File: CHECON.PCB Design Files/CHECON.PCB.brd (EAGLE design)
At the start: 81.7 x 51.6 mm, 73 parts

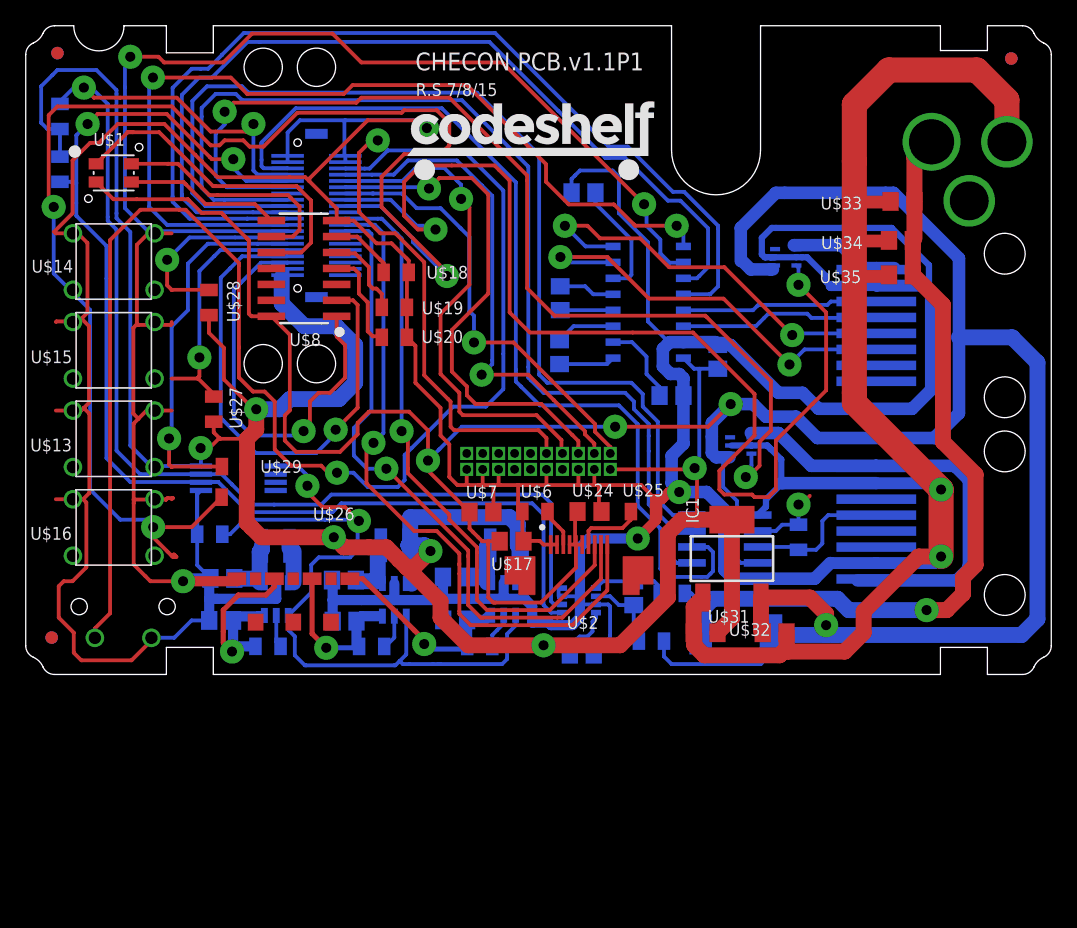
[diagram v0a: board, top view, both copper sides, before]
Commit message: New CHE
Starting on new CHE
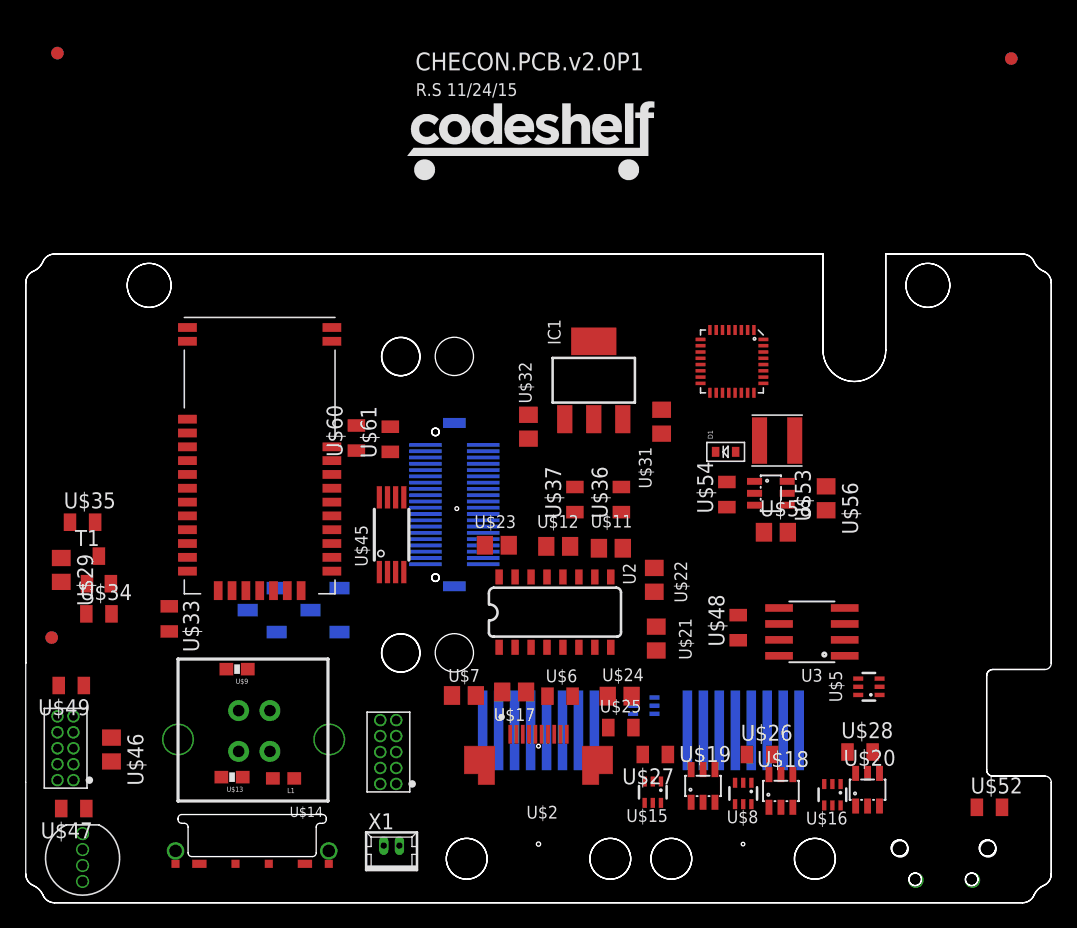
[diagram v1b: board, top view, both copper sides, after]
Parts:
- removed C11, C14: 0.1uF, GW-devices:C0805
- removed LQH3NPN100NM0L: 1212_IND, KW2:1212_IND
- removed R10: (no value), GW-devices:R2512
- removed R12, R13: 10, GW-devices:RF-C0805
- removed U$59: BL_CON, KW2:009155004301006
- removed U$62: INA219B, KW2:DCN-R-PDSO-G8
- added D1: (no value), adafruit:SOD-523
- added JP1, JP2: (no value), KW2:2X5HDR
- added L1: (no value), SparkFun:0603
- added T1: BC849, transistor:SOT23
- added X1: 53047-02, con-molex:53047-02
- U$1: value RGLBED -> 2.7_BL_CONN; device KW2:RGBLED -> KW2:XD2B-0406-26A
- U$13: value SWITCH-TACTILE-FSM -> TVS0603; device GW-devices:SWITCH-TACTILE-FSM -> SparkFun:0603-RES
- U$14: value SWITCH-TACTILE-FSM -> USB_B; device GW-devices:SWITCH-TACTILE-FSM -> KW2:USB-B-PTH-VERTICAL
- U$15, U$16: value SWITCH-TACTILE-FSM -> MIC94061C6; device GW-devices:SWITCH-TACTILE-FSM -> GW-devices:SC70-6L
- U$18, U$19, U$20: value 24 -> BCR401U; device GW-devices:RF-C0805 -> KW2:SOT23-6
- U$26: value 10k -> 40
- U$27, U$28: value 10k -> 15
- U$29: value 10k -> 220pF; device GW-devices:RF-C0805 -> GW-devices:C0805
- U$3: value 2X10JTAG -> KL20; device KW2:2X10JTAG -> KW2:QFN-32
- U$33: value 0.1uF -> 1.5k; device GW-devices:C0805 -> GW-devices:RF-C0805
- U$34: value 1uF -> 4.7k; device GW-devices:C0805 -> GW-devices:RF-C0805
- U$35: value 10uF -> 1.1k; device GW-devices:C0805 -> GW-devices:RF-C0805
- U$36, U$37: value SC4541 -> 10k; device KW2:SOT23-6 -> GW-devices:RF-C0805
- U$4, U$5: value (none) -> MIC94061C6
- U$44: value SC4541 -> LED_PTH_2812; device KW2:SOT23-6 -> KW2:LED_PTH_2812
- U$46: value 10k -> 0.1uF; device GW-devices:RF-C0805 -> GW-devices:C0805
- U$47, U$49: value 1212_IND -> 10k; device KW2:1212_IND -> GW-devices:RF-C0805
- U$50, U$51: value 1uF -> CJS; device GW-devices:C0805 -> KW2:CJS
- U$52: value 1uF -> 10k; device GW-devices:C0805 -> GW-devices:RF-C0805
- U$53: value 1uF -> AP5724; device GW-devices:C0805 -> KW2:SOT23-6
- U$54: value 1uF -> 4.99; device GW-devices:C0805 -> GW-devices:RF-C0805
- U$55: value 1uF -> NR4012T220M; device GW-devices:C0805 -> KW2:NR4012T220M
- U$56: value 6.8 -> 1uF; device GW-devices:RF-C0805 -> GW-devices:C0805
- U$57: value 3.3 -> BM78; device GW-devices:RF-C0805 -> KW2:BM78
- U$58: value 3.3 -> 1uF; device GW-devices:RF-C0805 -> GW-devices:C0805
- U$8: value (none) -> MIC94061C6; device GW-devices:SO14 -> GW-devices:SC70-6L
- U$9: value BARREL_CUI_PJ-002A -> TVS0603; device KW2:BARREL_CUI_PJ-002A -> SparkFun:0603-RES
- U2: value (none) -> MAX232SOIC16
- U3: value (none) -> RS485SOIC
- moved U$34 70.4 mm to (-35.0, -21.0)
- moved U$9 69.4 mm to (-24.0, -25.4), flipped to the top
- moved U$30 68.2 mm to (32.3, -42.2)
- moved U$35 68.1 mm to (-36.3, -13.7)
- moved U$33 67.2 mm to (-29.4, -21.4), turned to 270 degrees
- moved U$28 63.0 mm to (25.6, -32.0), turned to 0 degrees
- moved U$16 61.0 mm to (23.4, -35.4), turned to 180 degrees
- moved SCANNER 56.4 mm to (0.00, -40.5), turned to 0 degrees
- moved U$1 56.1 mm to (-22.8, -40.9), turned to 0 degrees
- moved U$15 55.5 mm to (9.10, -35.2), turned to 180 degrees
- moved U$8 54.5 mm to (16.3, -35.3), turned to 180 degrees
- moved U$20 52.1 mm to (26.2, -35.0)
- moved U$18 51.4 mm to (19.3, -35.1)
- moved U$26 46.6 mm to (17.6, -32.2)
- moved U$55 46.5 mm to (19.0, -7.20), flipped to the top, turned to 180 degrees
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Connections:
- removed net N$24: POSCON.P$1, POSCON.P$8, U$5.1
- new net +5V: IC1.3, U$15.4, U$16.4, U$31.2, U$44.P$2, U$8.4
- new net N$58: JP2.P$10, U$3.19, U$49.2
- net +3V3: now also JP1.P$1, JP2.P$1, U$36.2, U$37.2, U$46.2, U$47.1, U$49.1, U$52.1, U$53.6, U$55.P$2, U$58.2; no longer C14.1, LQH3NPN100NM0L.P$1, U$21.1, U$26.2, U$27.2, U$28.2, U$29.2, U$3.P$1, U$36.3, U$37.3, U$44.3, U$47.P$1, U$49.P$1, U$62.4, U2.16
- net GND: now also JP1.P$3, JP1.P$5, JP2.P$3, JP2.P$5, L1.2, U$1.P$4, U$13.1, U$14.GND, U$15.2, U$15.5, U$16.2, U$16.5, U$18.1, U$19.1, U$20.1, U$29.1, U$44.P$3, U$56.1, U$57.P$1, U$57.P$2, U$57.P$3, U$57.P$31, U$57.P$32, U$57.P$33, U$58.1, U$8.2, U$8.5, U$9.1; no longer C14.2, U$13.P$1, U$13.P$2, U$14.P$1, U$14.P$2, U$15.P$1, U$15.P$2, U$16.P$1, U$16.P$2, U$18.2, U$19.2, U$20.2, U$3.P$15, U$3.P$17, U$3.P$19, U$3.P$3, U$3.P$5, U$3.P$9, U$33.1, U$34.1, U$36.2, U$37.2, U$44.2, U$50.1, U$51.1, U$52.1, U$55.2, U$59.P$4, U$62.3, U$62.7, U$62.8, U$8.7, U$9.P$2
- net N$1: now also JP1.P$2, U$50.P$1; no longer U$3.P$2
- net N$11: now also U$33.2, U$34.2; no longer U$8.1
- net N$13: now also U$16.1, U$20.4, U$28.1; no longer U$18.1, U$8.6
- net N$14: now also U$15.1, U$19.4, U$27.1; no longer U$19.1, U$8.5
- net N$15: now also U$18.4, U$26.1, U$8.1; no longer U$20.1, U$8.4
- net N$16: now also T1.2; no longer U$8.2
- net N$2: now also U$45.2, U$53.4; no longer U$10.P$12, U$3.P$6
- net N$25: now also U$21.1, U2.16
- net N$3: now also U$53.3, U$54.1, X1.2; no longer U$10.P$10, U$3.P$8
- net N$35: now also U$14.D-, U$3.4, U$9.2; no longer U$10.P$31, U$15.P$4, U$27.1
- net N$36: now also U$13.2, U$14.D+, U$3.3; no longer U$10.P$27, U$14.P$4, U$28.1
- net N$37: now also U$20.6, U$28.2; no longer U$10.P$29, U$13.P$4, U$29.1
- net N$39: now also U$36.1
- net N$4: now also JP1.P$4, U$51.P$1; no longer U$3.P$4
- net N$40: now also U$37.1
- net N$42: now also U$19.6, U$27.2; no longer U$10.P$18, U$16.P$4, U$26.1
- net N$43: now also U$18.6, U$26.2; no longer U$36.4, U$37.4, U$44.4, U$45.1, U$46.2
- net N$44: now also U$16.3, U$45.1, U$8.3; no longer U$37.1, U$47.P$2, U$50.2
- net N$45: no longer U$62.6
- net N$46: now also U$10.P$18; no longer LQH3NPN100NM0L.P$2, U$36.1, U$52.2
- net N$47: no longer U$62.5
- net N$48: now also T1.3, U$33.1, U$44.P$1; no longer U$44.1, U$49.P$2, U$51.2
- net N$49: now also T1.1, U$29.2, U$34.1; no longer R10.1, R12.2, U$33.2, U$34.2, U$9.P$1
- net N$5: now also L1.1, U$14.P$1, U$14.P$2; no longer U$1.P$4, U$8.9
- net N$50: now also D1.A, U$53.1, U$55.P$1; no longer U$44.5, U$58.2
- net N$51: now also U$1.P$3, U$20.2, U$20.3, U$20.5; no longer U$44.6, U$55.1, U$58.1, U$59.P$3
- net N$52: now also JP2.P$2, U$3.15, U$47.2; no longer U$37.5, U$57.2
- net N$53: now also U$1.P$2, U$19.2, U$19.3, U$19.5; no longer U$37.6, U$54.1, U$57.1, U$59.P$2
- net N$54: now also D1.K, U$53.5, U$56.2, X1.1; no longer U$36.6, U$53.1, U$56.1, U$59.P$1
- net N$55: now also JP2.P$4, U$3.12; no longer U$36.5, U$56.2
- net N$56: now also JP2.P$6, U$3.14; no longer C11.1, R12.1, U$62.1
- net N$57: now also JP2.P$8, U$3.13; no longer C11.2, R13.1, U$62.2
- net N$6: now also JP1.P$10, U$3.21, U$52.2; no longer U$3.P$10
- net N$8: now also U$15.3; no longer U$1.P$3, U$8.8
- net N$9: now also U$18.2, U$18.3, U$18.5; no longer U$8.10
- net V+: now also POSCON.P$1, POSCON.P$8, U$5.1; no longer IC1.3, R10.2, R13.2, U$1.P$2, U$31.2, U$8.14
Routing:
- net GND: track 554.5 -> 0.00 mm, vias 6 -> 0
- net V+: track 252.5 -> 0.00 mm, vias 4 -> 0
- net +3V3: track 218.0 -> 0.00 mm, vias 6 -> 0
- net N$6: track 153.7 -> 0.00 mm, vias 2 -> 0
- net N$42: track 112.1 -> 0.00 mm, vias 3 -> 0
- net N$45: track 100.4 -> 0.00 mm, vias 2 -> 0
- net N$47: track 95.8 -> 0.00 mm, vias 2 -> 0
- net N$40: track 90.2 -> 0.00 mm, vias 2 -> 0
- net N$27: track 84.3 -> 0.00 mm
- net N$17: track 83.9 -> 0.00 mm
- net N$39: track 80.7 -> 0.00 mm, vias 2 -> 0
- net N$41: track 80.2 -> 0.00 mm, vias 2 -> 0
- net N$10: track 78.2 -> 0.00 mm
- net N$28: track 76.7 -> 0.00 mm
- net N$26: track 72.3 -> 0.00 mm
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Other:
- outline, holes or cut-outs redrawn
- board text added: "CHECON.PCB.v2.0P1"
- board text added: "R.S 11/24/15"
- board text removed: "CHECON.PCB.v1.1P1"
- board text removed: "R.S 7/8/15"
